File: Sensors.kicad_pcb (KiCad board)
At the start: 4 copper layers, 20.8 x 14.3 mm, 10 parts, among them J1 Conn_01x06_Male, U01 BMI270, U02 BMM150

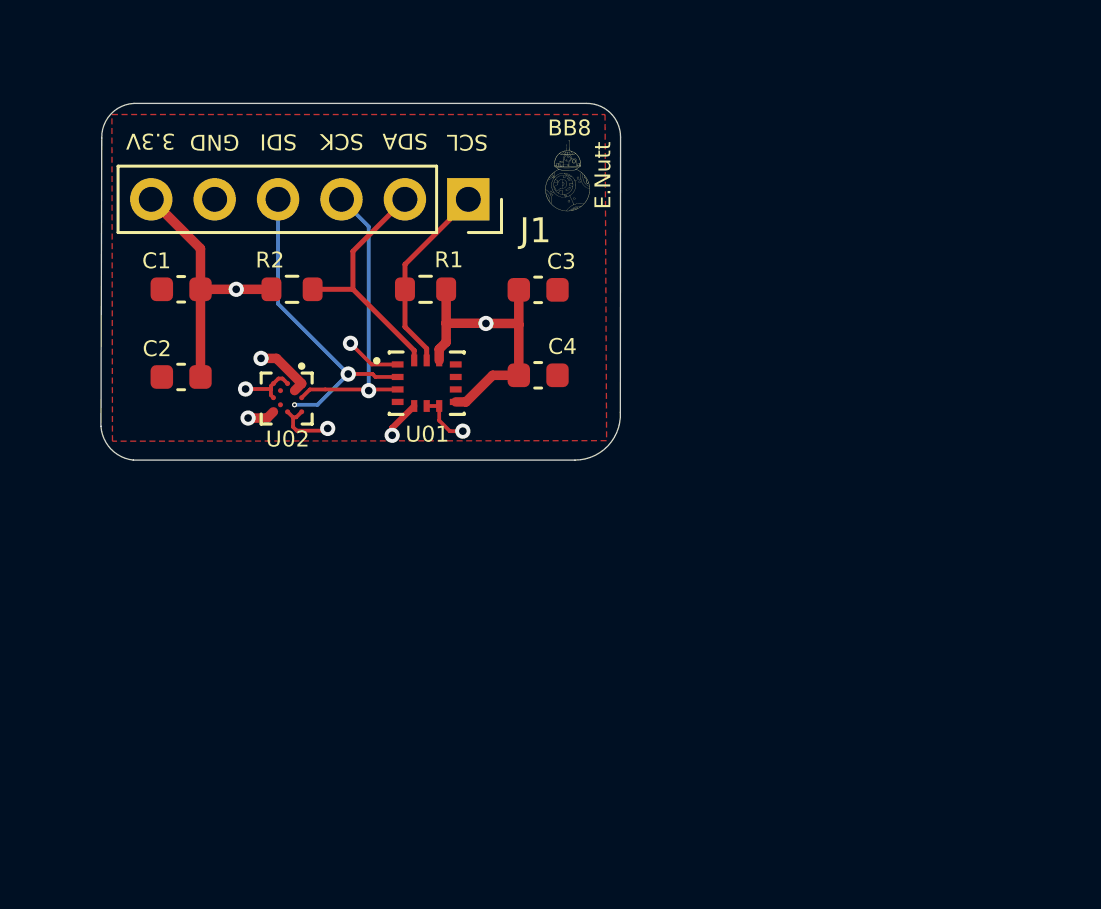
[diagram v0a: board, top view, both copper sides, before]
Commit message: biggie cheese
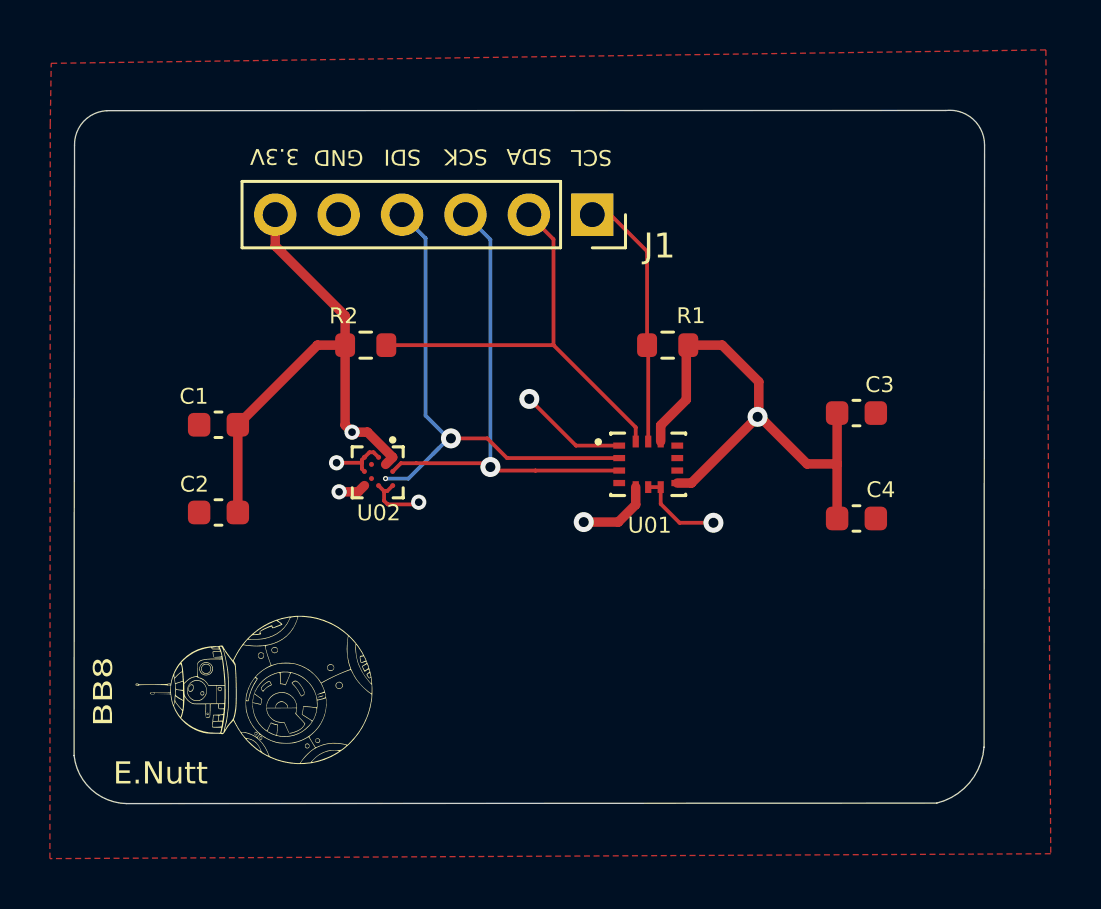
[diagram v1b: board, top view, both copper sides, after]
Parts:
- moved G*** 24.1 mm to (93.2, 68.6), turned to 90 degrees
- moved C4 14.0 mm to (117.4, 61.7)
- moved C3 13.7 mm to (117.4, 57.5)
- moved R1 9.95 mm to (109.8, 54.7)
- moved U01 9.45 mm to (109.0, 59.5)
- moved C1 5.63 mm to (91.8, 57.9)
- moved C2 5.63 mm to (91.8, 61.4)
- moved J1 5.00 mm to (106.8, 49.5)
- moved U02 4.69 mm to (98.2, 59.8)
- moved R2 3.70 mm to (97.7, 54.7)
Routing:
- net 3.3V: track 28.3 -> 47.4 mm, vias 5 -> 4
- net Net-(U01-Pad3): track 12.1 -> 19.9 mm
- net Net-(U01-Pad2): track 12.9 -> 20.5 mm
- net Net-(U01-Pad14): track 10.2 -> 17.6 mm
- net GND: track 9.50 -> 13.0 mm
- net Net-(U01-Pad13): track 8.02 -> 10.4 mm
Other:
- board size 20.8 x 14.3 mm -> 36.5 x 27.8 mm
